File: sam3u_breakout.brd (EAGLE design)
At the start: 57.9 x 44.6 mm, 26 parts, among them IC1 SAM3U_LQFP100

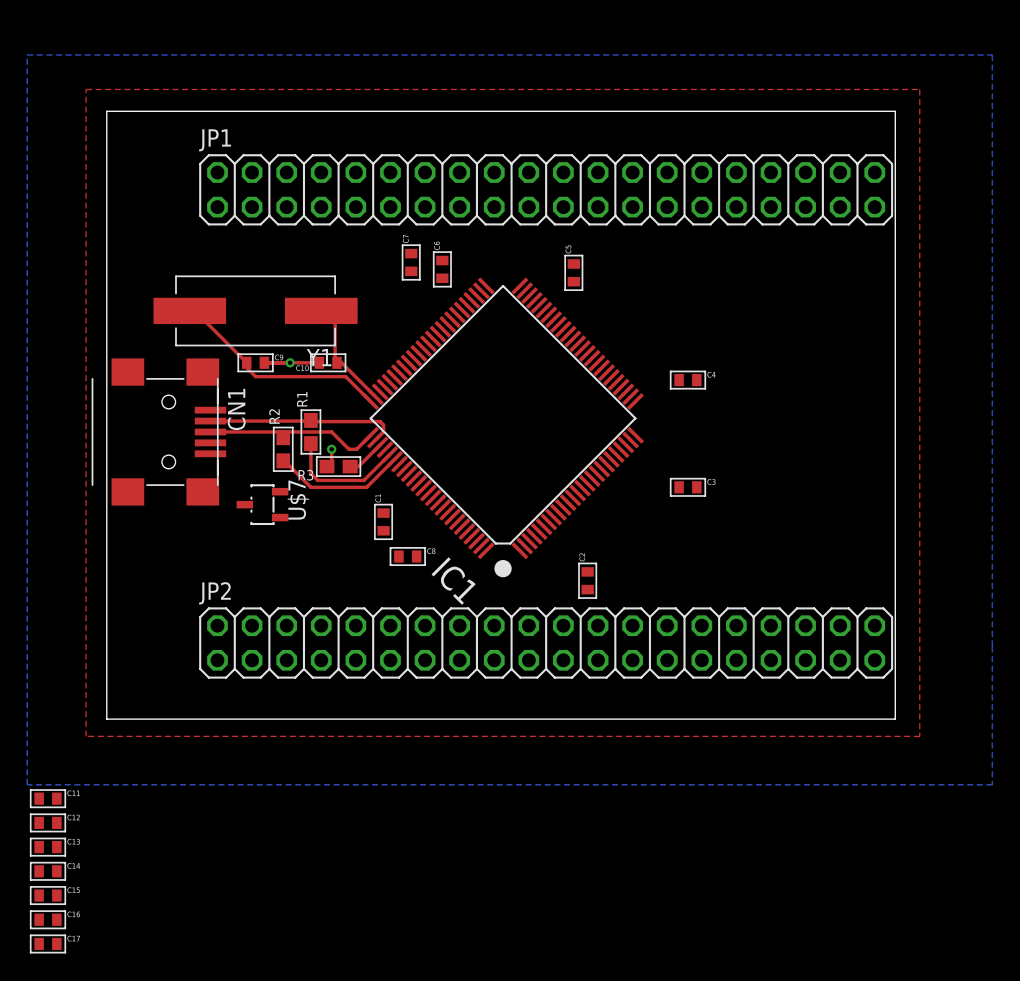
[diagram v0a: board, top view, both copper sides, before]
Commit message: Route board
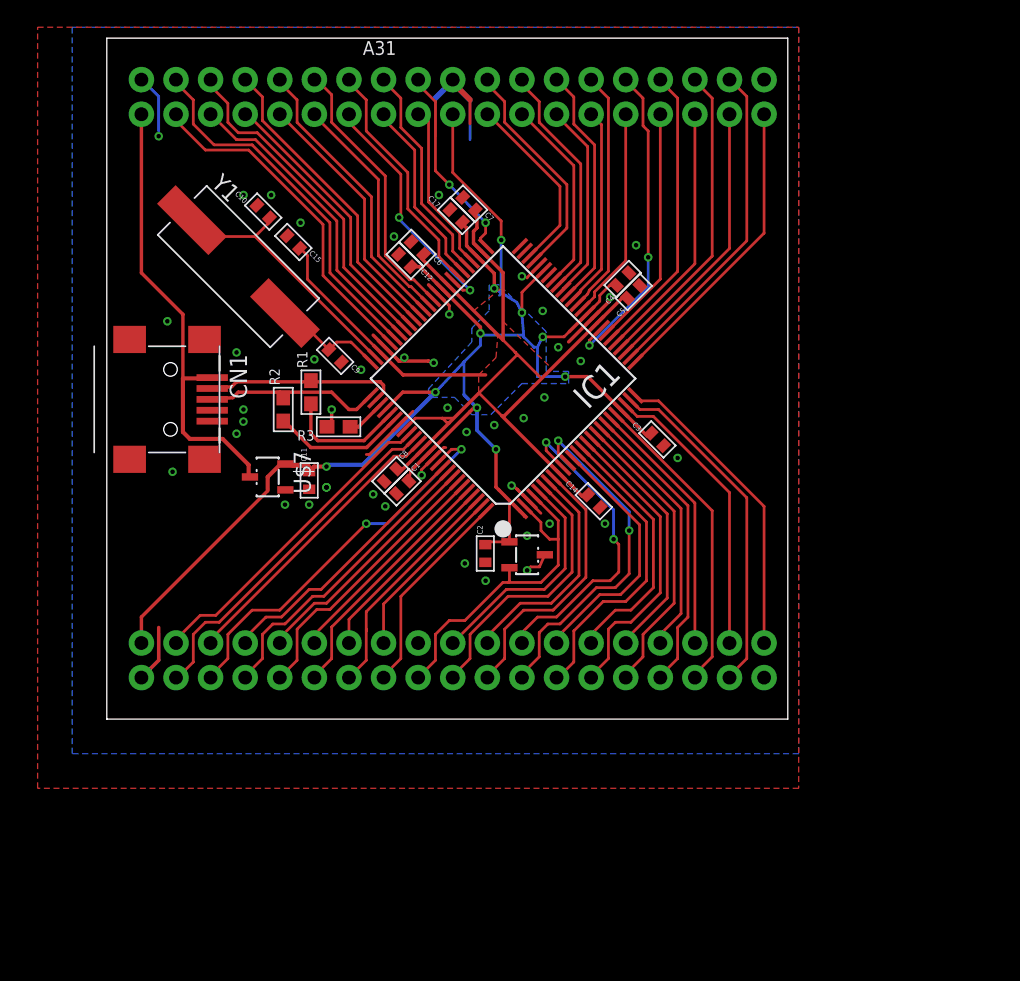
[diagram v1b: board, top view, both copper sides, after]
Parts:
- removed C13, C16: (no value), nonolith:0402
- removed JP1, JP2: (no value), adafruit:2X20
- added U$10, U$11, U$12, U$13: M191X19_NO_SILK, SparkFun-Connectors:1X19_NO_SILK
- added U$14: VREF, nonolith:SOT23-3
- moved C17 61.3 mm to (25.7, 36.9), turned to 135 degrees
- moved C15 51.3 mm to (13.7, 35.0), turned to 315 degrees
- moved C12 48.9 mm to (21.9, 33.7), turned to 315 degrees
- moved C14 48.4 mm to (35.8, 16.0), turned to 135 degrees
- moved C11 30.2 mm to (14.9, 17.5), turned to 90 degrees
- moved C10 12.1 mm to (11.5, 37.3), turned to 135 degrees
- moved C4 8.83 mm to (37.9, 32.3), turned to 225 degrees
- moved C2 7.78 mm to (27.8, 12.2)
- moved C8 6.10 mm to (20.8, 17.9), turned to 45 degrees
- moved C7 6.05 mm to (26.6, 37.8), turned to 315 degrees
- moved C9 5.86 mm to (16.8, 26.7), turned to 315 degrees
- moved C5 4.61 mm to (38.7, 31.4), turned to 225 degrees
- moved C3 4.18 mm to (40.4, 20.5), turned to 135 degrees
- moved Y1 3.49 mm to (9.67, 33.2), turned to 315 degrees
- moved IC1 2.92 mm to (29.1, 25.0)
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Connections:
- removed net N$3: C14.2, C15.2, C16.2, C5.2, C6.2, C7.2, C8.2, IC1.34, IC1.52, IC1.59, IC1.73, IC1.83, IC1.87, IC1.9
- new net 1.8V: C14.2, C15.2, C5.2, C6.2, C7.2, C8.2, IC1.34, IC1.52, IC1.59, IC1.73, IC1.83, IC1.87, IC1.9
- new net ERASE: IC1.43, U$11.12
- new net FWUP: IC1.42, U$10.12
- new net JTAGSEL: IC1.48, U$11.11
- new net N$17: IC1.49
- new net N$18: IC1.50
- new net NRST: IC1.57, U$10.7
- new net NRSTB: IC1.47, U$10.11
- new net PA0: IC1.26, U$11.19
- new net PA1: IC1.27, U$10.18
- new net PA10: IC1.39, U$11.14
- new net PA11: IC1.40, U$10.13
- new net PA12: IC1.41, U$11.13
- new net PA13: IC1.10, U$13.12
- new net PA14: IC1.11, U$12.12
- new net PA15: IC1.12, U$13.13
- new net PA16: IC1.13, U$12.13
- new net PA17: IC1.14, U$13.14
- new net PA18: IC1.17, U$12.15
- new net PA19: IC1.18, U$13.16
- new net PA2: IC1.28, U$11.18
- new net PA20: IC1.19, U$12.16
- new net PA21: IC1.20, U$13.17
- new net PA22: IC1.5, U$13.10
- new net PA23: IC1.21, U$12.17
- new net PA24: IC1.23, U$13.18
- new net PA25: IC1.24, U$12.18
- new net PA26: IC1.25, U$13.19
- new net PA27: IC1.96, U$12.6
- new net PA28: IC1.84, U$13.2
- new net PA29: IC1.85, U$12.2
- new net PA3: IC1.29, U$10.17
- new net PA30: IC1.6, U$12.10
- new net PA31: IC1.86, U$13.3
- new net PA4: IC1.30, U$11.17
- new net PA5: IC1.31, U$10.16
- new net PA6: IC1.32, U$11.16
- new net PA7: IC1.33, U$10.15
- new net PA8: IC1.37, U$11.15
- new net PA9: IC1.38, U$10.14
- new net PB0: IC1.90, U$12.3
- new net PB1: IC1.91, U$13.4
- new net PB10: IC1.70, U$10.2
- new net PB11: IC1.93, U$13.5
- new net PB12: IC1.94, U$12.5
- new net PB13: IC1.95, U$13.6
- new net PB14: IC1.69, U$11.3
- new net PB15: IC1.16, U$13.15
- new net PB16: IC1.15, U$12.14
- new net PB17: IC1.68, U$10.3
- new net PB18: IC1.67, U$11.4
- new net PB19: IC1.66, U$10.4
- new net PB2: IC1.92, U$12.4
- new net PB20: IC1.65, U$11.5
- new net PB21: IC1.64, U$10.5
- new net PB22: IC1.63, U$11.6
- new net PB23: IC1.62, U$10.6
- new net PB24: IC1.58, U$11.7
- new net PB3: IC1.7, U$13.11
- new net PB4: IC1.8, U$12.11
- new net PB5: IC1.97, U$13.7
- new net PB6: IC1.98, U$12.7
- new net PB7: IC1.99, U$13.8
- new net PB8: IC1.100, U$12.8
- new net PB9: IC1.71, U$11.2
- new net TCK: IC1.56, U$11.8
- new net TDI: IC1.51, U$10.9
- new net TDO: IC1.54, U$11.9
- new net TMS: IC1.55, U$10.8
- new net TST: IC1.44
- net 3.3V: now also U$11.10, U$13.1, U$14.1; no longer C13.2
- net 5V: now also U$11.1
- net ADVREF: now also IC1.4, U$12.9, U$14.2
- net GND: now also U$10.1, U$10.10, U$10.19, U$12.1, U$12.19, U$13.9, U$14.3; no longer C13.1, C16.1
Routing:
- net 3.3V: track 0.00 -> 132.0 mm, vias 0 -> 10
- net 1.8V: track 0.00 -> 83.2 mm
- net GND: track 7.34 -> 56.3 mm, vias 2 -> 44
- net 5V: track 0.00 -> 33.5 mm
- net PB0: track 0.00 -> 28.6 mm, vias 0 -> 2
- net PB10: track 0.00 -> 27.2 mm
- net PA14: track 0.00 -> 26.1 mm, vias 0 -> 2
- net PA29: track 0.00 -> 25.9 mm
- net ADVREF: track 0.00 -> 25.5 mm
- net PA25: track 0.00 -> 25.2 mm
- net PB9: track 0.00 -> 25.1 mm
- net PB17: track 0.00 -> 24.9 mm
- net PA1: track 0.00 -> 24.4 mm
- net PA13: track 0.00 -> 23.8 mm, vias 0 -> 2
- net PA7: track 0.00 -> 23.7 mm, vias 0 -> 2
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- added copper zone on layer 1, net 1.8V
- added copper zone on layer 16, net 3.3V
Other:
- board size 57.9 x 44.6 mm -> 50 x 50 mm
- board text added: "A31"
